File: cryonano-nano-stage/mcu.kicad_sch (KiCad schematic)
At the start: 2 parts, among them U1 2DIB0410FXUMA1, U2 2DIB1410FXUMA1

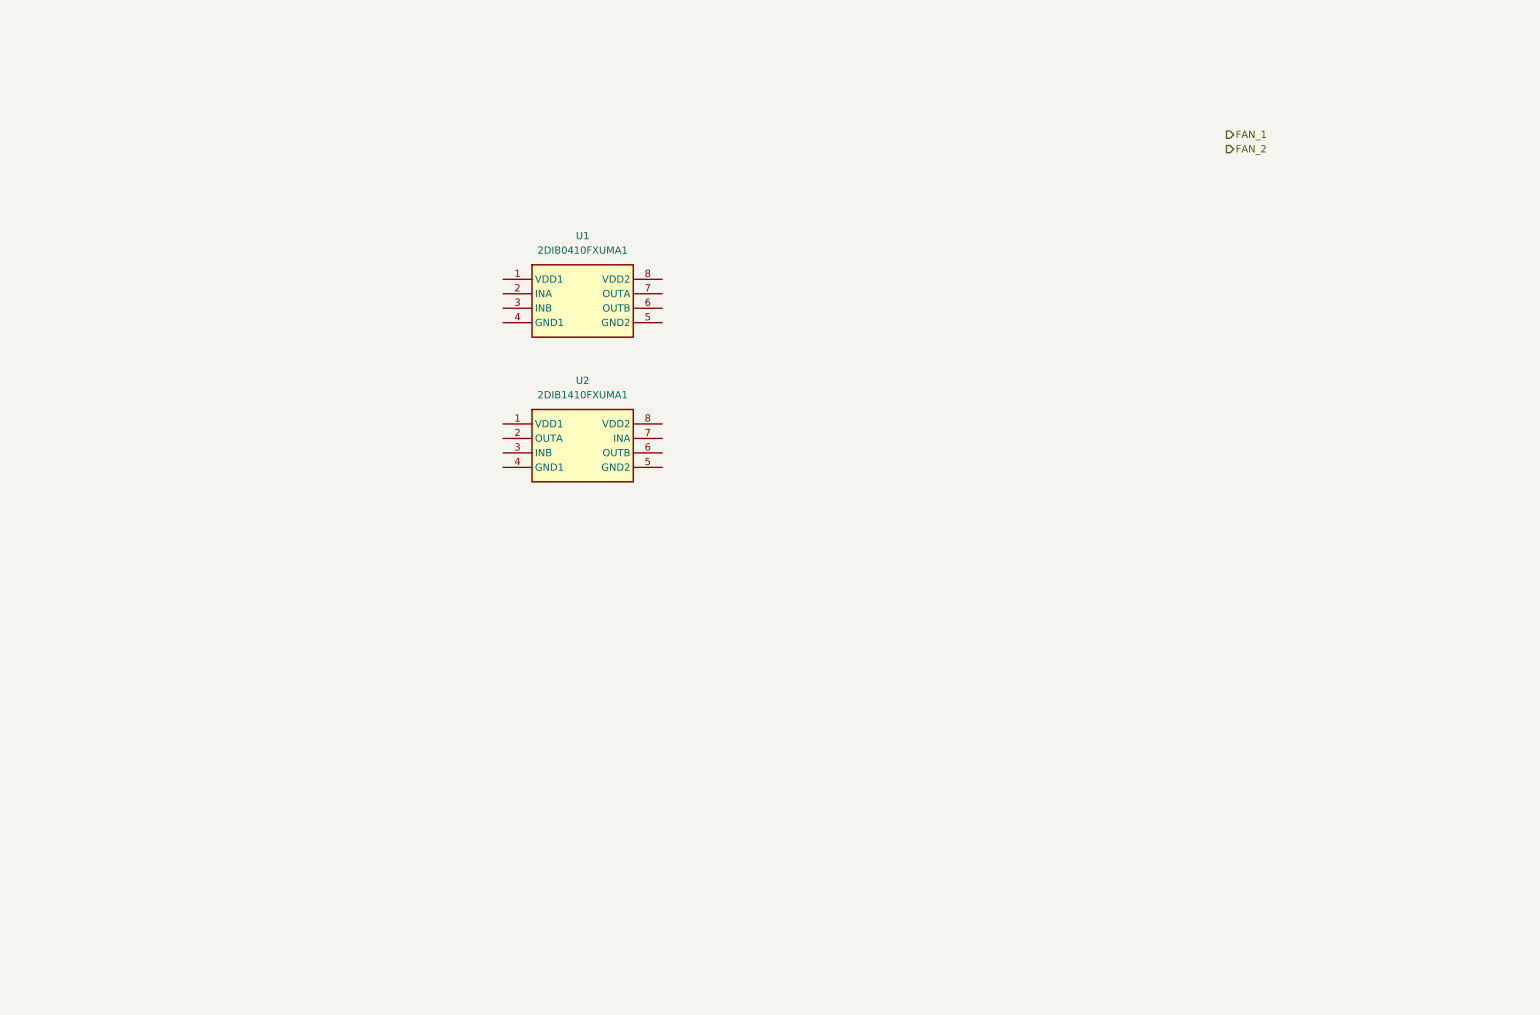
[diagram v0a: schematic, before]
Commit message: preliminary components added
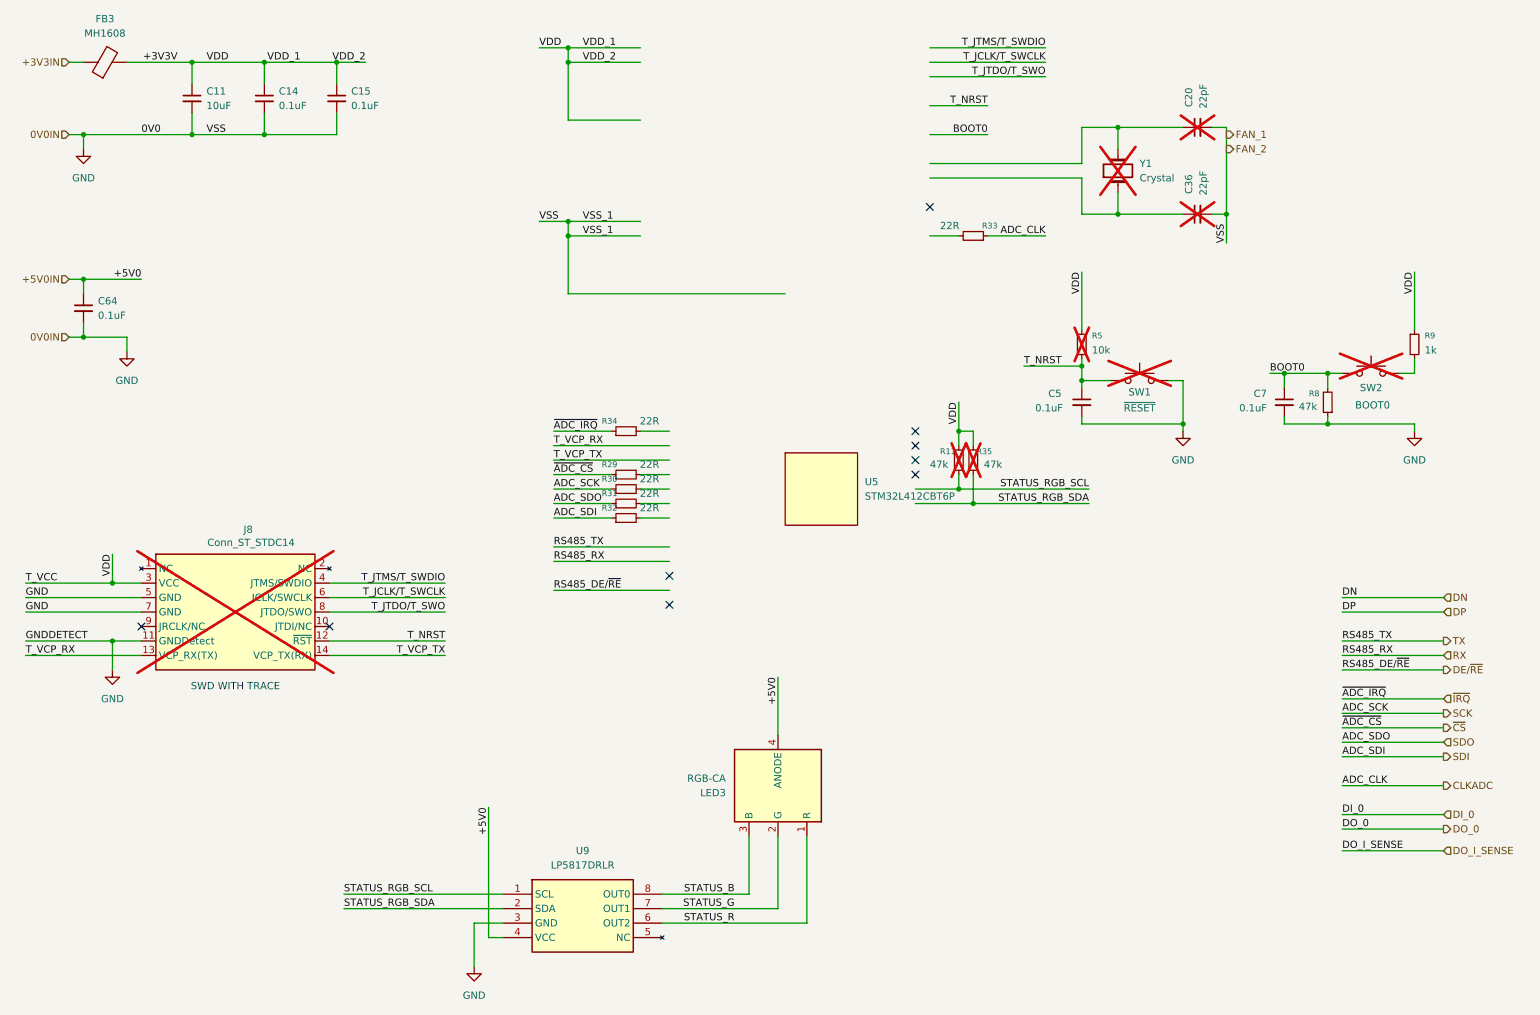
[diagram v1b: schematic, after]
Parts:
- removed U1: 2DIB0410FXUMA1, SOIC127P600X175-8N, symbol symbols:2DIB0410FXUMA1
- removed U2: 2DIB1410FXUMA1, SOIC127P600X175-8N, symbol symbols:2DIB1410FXUMA1
- added C11: 10uF, Capacitor_SMD:C_0805_2012Metric, symbol Device:C_Small
- added C14, C15, C5, C64, C7: 0.1uF, Capacitor_SMD:C_0603_1608Metric, symbol Device:C_Small
- added C20, C36: 22pF, Capacitor_SMD:C_0603_1608Metric, symbol Device:C_Small
- added FB3: MH1608, Inductor_SMD:L_0603_1608Metric, symbol Device:FerriteBead
- added J8: Conn_ST_STDC14, footprints:PinHeader_2x07_P1.27mm_Vertical, symbol symbols:Conn_ST_STDC14
- added LED3: RGB-CA, footprints:19037ARSGHBHW1S032T, symbol symbols:19-037A_RSGHBHW1-S03_2T
- added R11, R35, R8: 47k, Resistor_SMD:R_0603_1608Metric, symbol Device:R_Small
- added R29, R30, R31, R32, R33, R34: 22R, Resistor_SMD:R_0603_1608Metric, symbol Device:R_Small
- added R5: 10k, Resistor_SMD:R_0603_1608Metric, symbol Device:R_Small
- added R9: 1k, Resistor_SMD:R_0603_1608Metric, symbol Device:R_Small
- added SW1: ~{RESET}, Button_Switch_SMD:SW_Tactile_SPST_NO_Straight_CK_PTS636Sx25SMTRLFS, symbol Switch:SW_Push
- added SW2: BOOT0, Button_Switch_SMD:SW_Tactile_SPST_NO_Straight_CK_PTS636Sx25SMTRLFS, symbol Switch:SW_Push
- added U5: STM32L412CBT6P, Package_QFP:LQFP-32_7x7mm_P0.8mm, symbol symbols:STM32L412CBT6P
- added U9: LP5817DRLR, footprints:LP5817DRLR, symbol symbols:LP5817DRLR
- added Y1: Crystal, Crystal:Crystal_SMD_3215-2Pin_3.2x1.5mm, symbol Device:Crystal
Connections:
- new net: R9.2, SW2.2
- new net: C36.1, Y1.1
- new net: C20.1, Y1.2
- new net +3V3IN: FB3.1
- new net +3V3V: C11.1, C14.1, C15.1, FB3.2, J8.3 (VCC), R11.2, R35.2, R5.1, R9.1
- new net +5V0IN: C64.1, LED3.4 (ANODE), U9.4 (VCC)
- new net BOOT0: C7.1, R8.2, SW2.1
- new net CLKADC: R33.1
- new net GND: C11.2, C14.2, C15.2, C20.2, C36.2, C5.2, C64.2, C7.2, J8.11 (GNDDetect), J8.5 (GND), J8.7 (GND), R8.1, SW1.2, U9.3 (GND)
- new net SCK: R30.1
- new net SDI: R32.1
- new net SDO: R31.1
- new net STATUS_B: LED3.3 (B), U9.8 (OUT0)
- new net STATUS_G: LED3.2 (G), U9.7 (OUT1)
- new net STATUS_R: LED3.1 (R), U9.6 (OUT2)
- new net STATUS_RGB_SCL: R11.1, U9.1 (SCL)
- new net STATUS_RGB_SDA: R35.1, U9.2 (SDA)
- new net T_JCLK/T_SWCLK: J8.6 (JCLK/SWCLK)
- new net T_JTDO/T_SWO: J8.8 (JTDO/SWO)
- new net T_JTMS/T_SWDIO : J8.4 (JTMS/SWDIO)
- new net T_NRST: C5.1, J8.12 (~{RST}), R5.2, SW1.1
- new net T_VCP_RX: J8.13 (VCP_RX(TX))
- new net T_VCP_TX: J8.14 (VCP_TX(RX))
- new net ~{CS}: R29.1
- new net ~{IRQ}: R34.1
- no-connect marks 0 -> 9
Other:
- note added: "SWD WITH TRACE"
